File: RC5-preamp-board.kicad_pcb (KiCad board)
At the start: 2 copper layers, 76.2 x 41.3 mm, 32 parts, among them P1 RAW_DC, P10 CTL_OUT, P2 VCC, P201 FTDI Basic, P3 VCC, P4 VCC, P5 VCC, P6 VCC, P8 INPUTS, P9 UI_OUT, SW201 Reset, U1 NCP1117DT50RKG, U201 ATMEGA328P-PU, U3 TSOP34136, X201 CSTLS16M0X53-B0

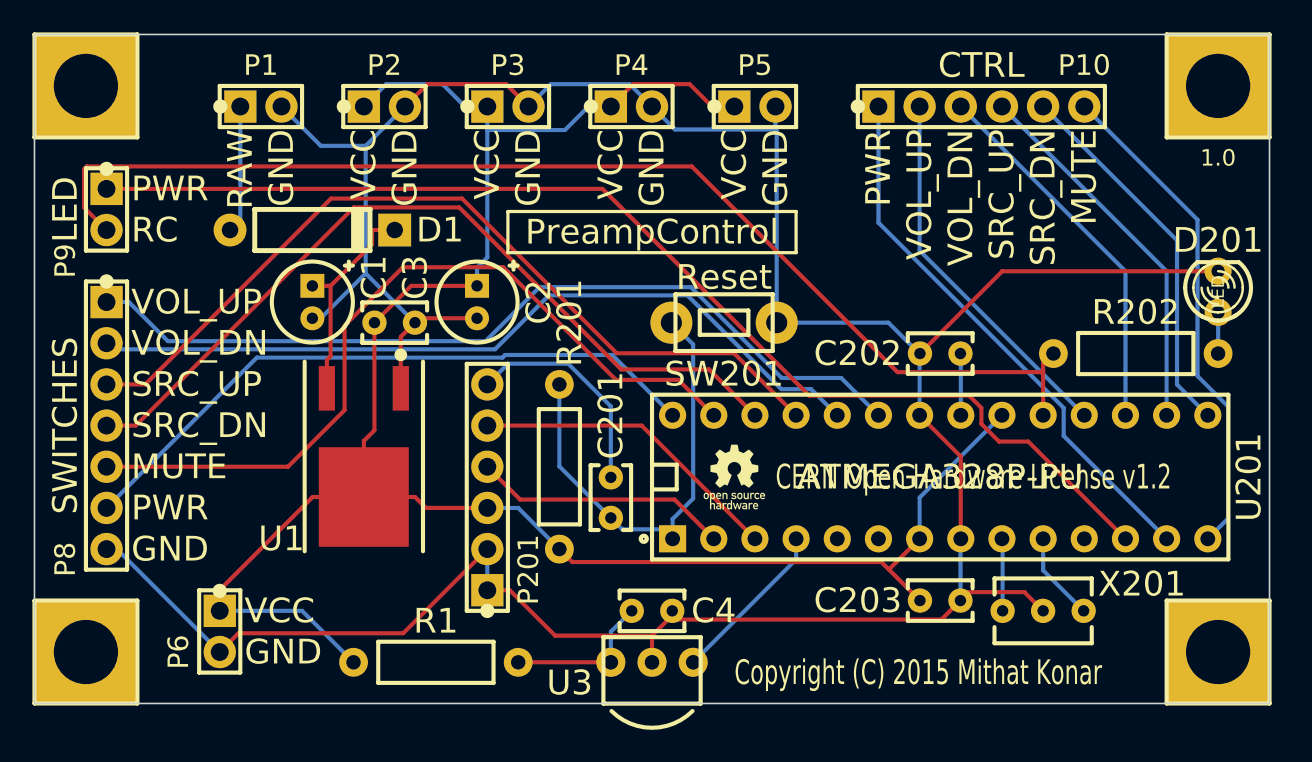
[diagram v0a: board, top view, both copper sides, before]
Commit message: Silk tweaks.
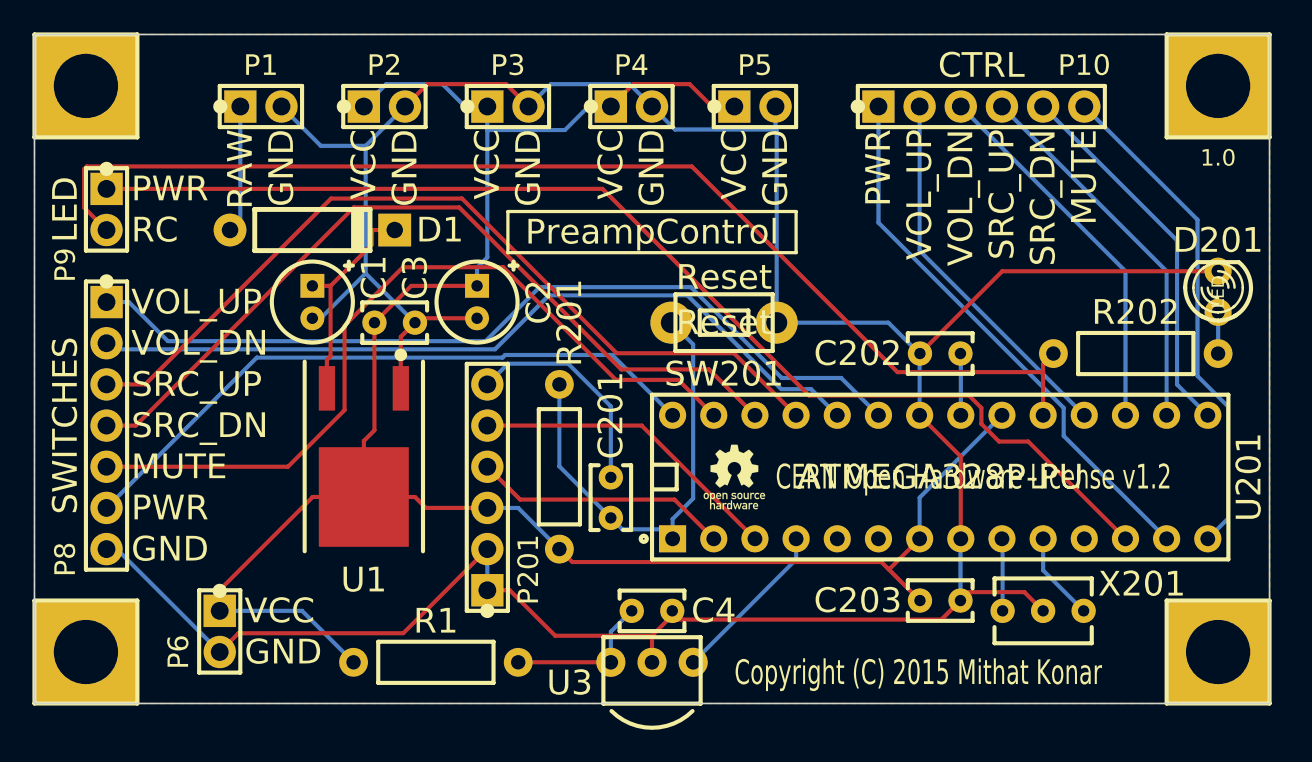
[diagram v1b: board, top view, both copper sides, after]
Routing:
- added copper zone on F.Cu, net DGND
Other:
- board text added: "Reset"
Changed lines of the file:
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@@
     (area 97.837172 76.099999 192.455715 147.48)
     (thickness 1.6)
-    (drawings 53)
+    (drawings 54)
     (tracks 205)
     (zones 0)
@@
     (visible_elements 7FFFFFFF)
     (pcbplotparams
-      (layerselection 3178497)
+      (layerselection 283148289)
       (usegerberextensions true)
       (excludeedgelayer true)
-      (linewidth 0.150000)
+      (linewidth 0.152400)
       (plotframeref false)
       (viasonmask false)
@@
       (psa4output false)
       (plotreference true)
-      (plotvalue true)
+      (plotvalue false)
       (plotothertext true)
       (plotinvisibletext false)
@@
       (outputformat 1)
       (mirror false)
-      (drillshape 1)
+      (drillshape 0)
       (scaleselection 1)
-      (outputdirectory ""))
+      (outputdirectory Gerbers))
   )
   (net 0 "")
@@
       (effects (font (size 1.524 1.524) (thickness 0.1524)))
     )
-    (fp_text value Reset (at 0 -2.794) (layer F.SilkS)
+    (fp_text value Reset (at 0 0) (layer F.SilkS)
       (effects (font (size 1.524 1.524) (thickness 0.1524)))
     )
@@
     (descr "2-pin SIL")
     (tags "CONN DEV SIL Jumper")
-    (fp_text reference P9 (at 3.175 2.54 270) (layer F.SilkS)
+    (fp_text reference P9 (at 3.429 2.54 270) (layer F.SilkS)
       (effects (font (size 1.27 1.27) (thickness 0.127)))
     )
@@
     (tags "DPAK TO-252 TO228P1003X238-3N IPC-7351")
     (attr smd)
-    (fp_text reference U1 (at 5.08 5.08 360) (layer F.SilkS)
+    (fp_text reference U1 (at 7.62 0 360) (layer F.SilkS)
       (effects (font (size 1.524 1.524) (thickness 0.1524)))
     )
@@
       (xy 1.47828 -0.47244)) (layer F.SilkS) (width 0.00254))
   )
+  (gr_text Reset (at 144.145 108.331) (layer F.SilkS)
+    (effects (font (size 1.524 1.524) (thickness 0.1524)))
+  )
   (gr_text "CERN Open Hardware License v1.2" (at 147.32 120.65) (layer F.SilkS)
     (effects (font (size 1.524 1.016) (thickness 0.254)) (justify left))
@@
   (segment (start 161.29 124.46) (end 161.33 124.5) (width 0.254) (layer B.Cu) (net 27))
   (segment (start 174.625 110.49) (end 174.625 113.03) (width 0.254) (layer B.Cu) (net 28))
+  (zone (net 23) (net_name DGND) (layer F.Cu) (hatch edge 0.508)
+    (connect_pads (clearance 0.508))
+    (min_thickness 0.2032)
+    (fill (arc_segments 16) (thermal_gap 0.508) (thermal_bridge_width 0.254))
+    (polygon
+      (pts
+        (xy 177.8 134.62) (xy 101.6 134.62) (xy 101.6 93.345) (xy 177.8 93.345)
+      )
+    )
+  )
 )
